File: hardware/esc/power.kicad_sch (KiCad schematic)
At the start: 34 parts, among them U13 TPS56339DDC, U14 NCP59800BMNADJTAG

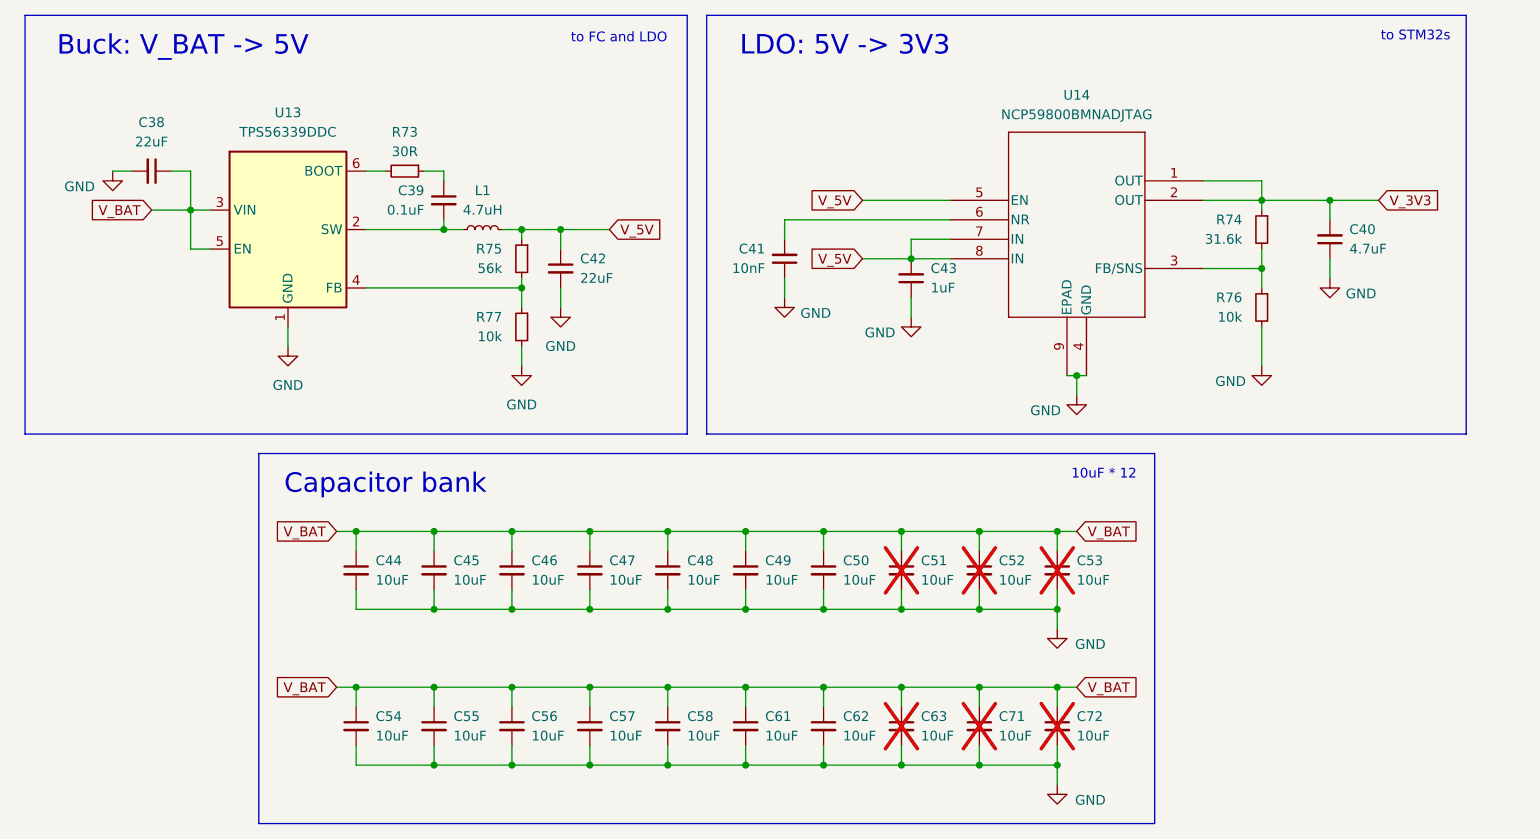
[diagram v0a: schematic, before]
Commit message: h/feat: power stage placement
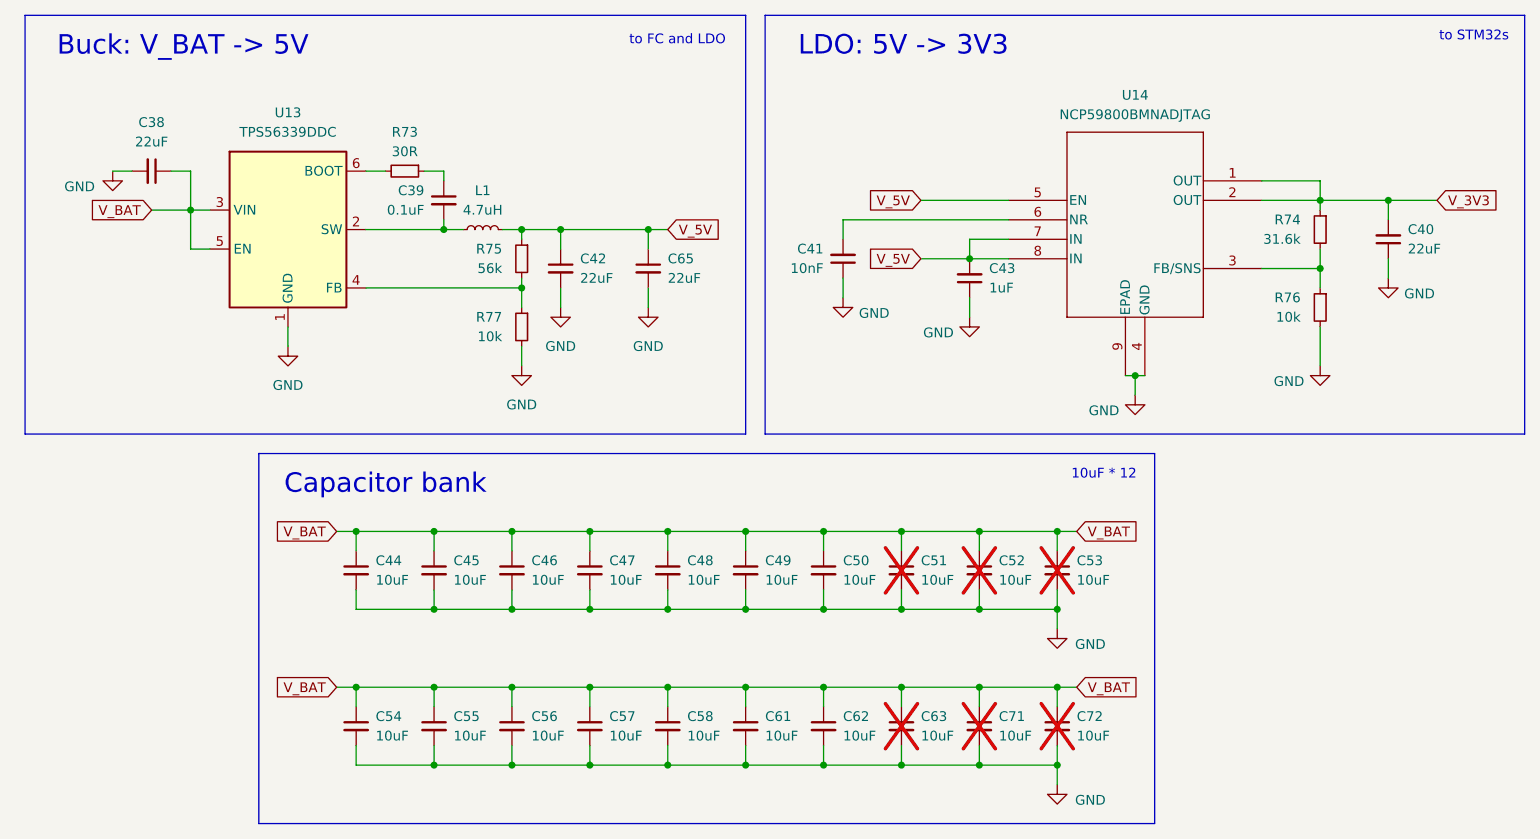
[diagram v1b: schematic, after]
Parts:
- added C65: 22uF, Capacitor_SMD:C_0805_2012Metric, symbol Device:C_Small
- C40: value 4.7uF -> 22uF; footprint Stratus:C_0402 -> Capacitor_SMD:C_0603_1608Metric
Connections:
- net GND: now also C65.2
- net V_5V: now also C65.1
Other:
- moved on the sheet: C40, C41, C43, R74, R76, U14
